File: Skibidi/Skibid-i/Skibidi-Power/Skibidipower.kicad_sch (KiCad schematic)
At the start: 19 parts, among them J1 SparkOut, J2 Bat2, J3 Bat1, J5 Sparkout 48V, J6 Sparkin, Q1 SQM40P10-40L_GE3, Q2 SQ2318AES-T1_BE3

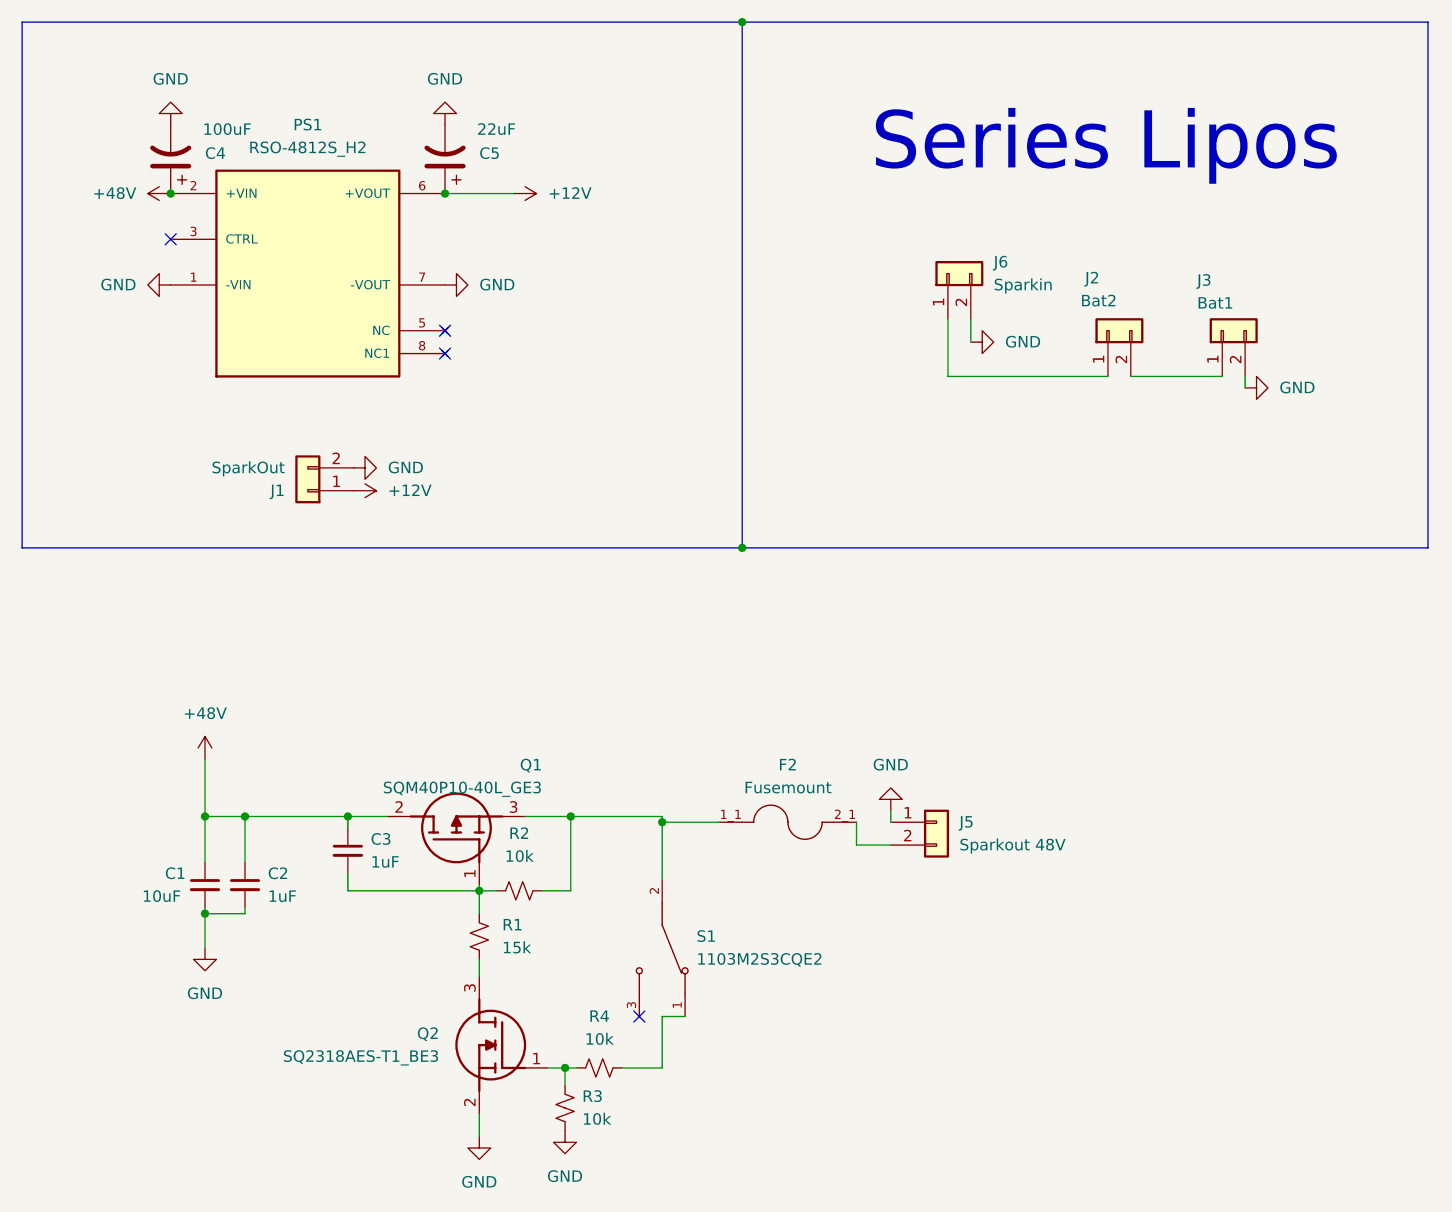
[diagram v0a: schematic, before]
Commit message: pushsuskibnbiid
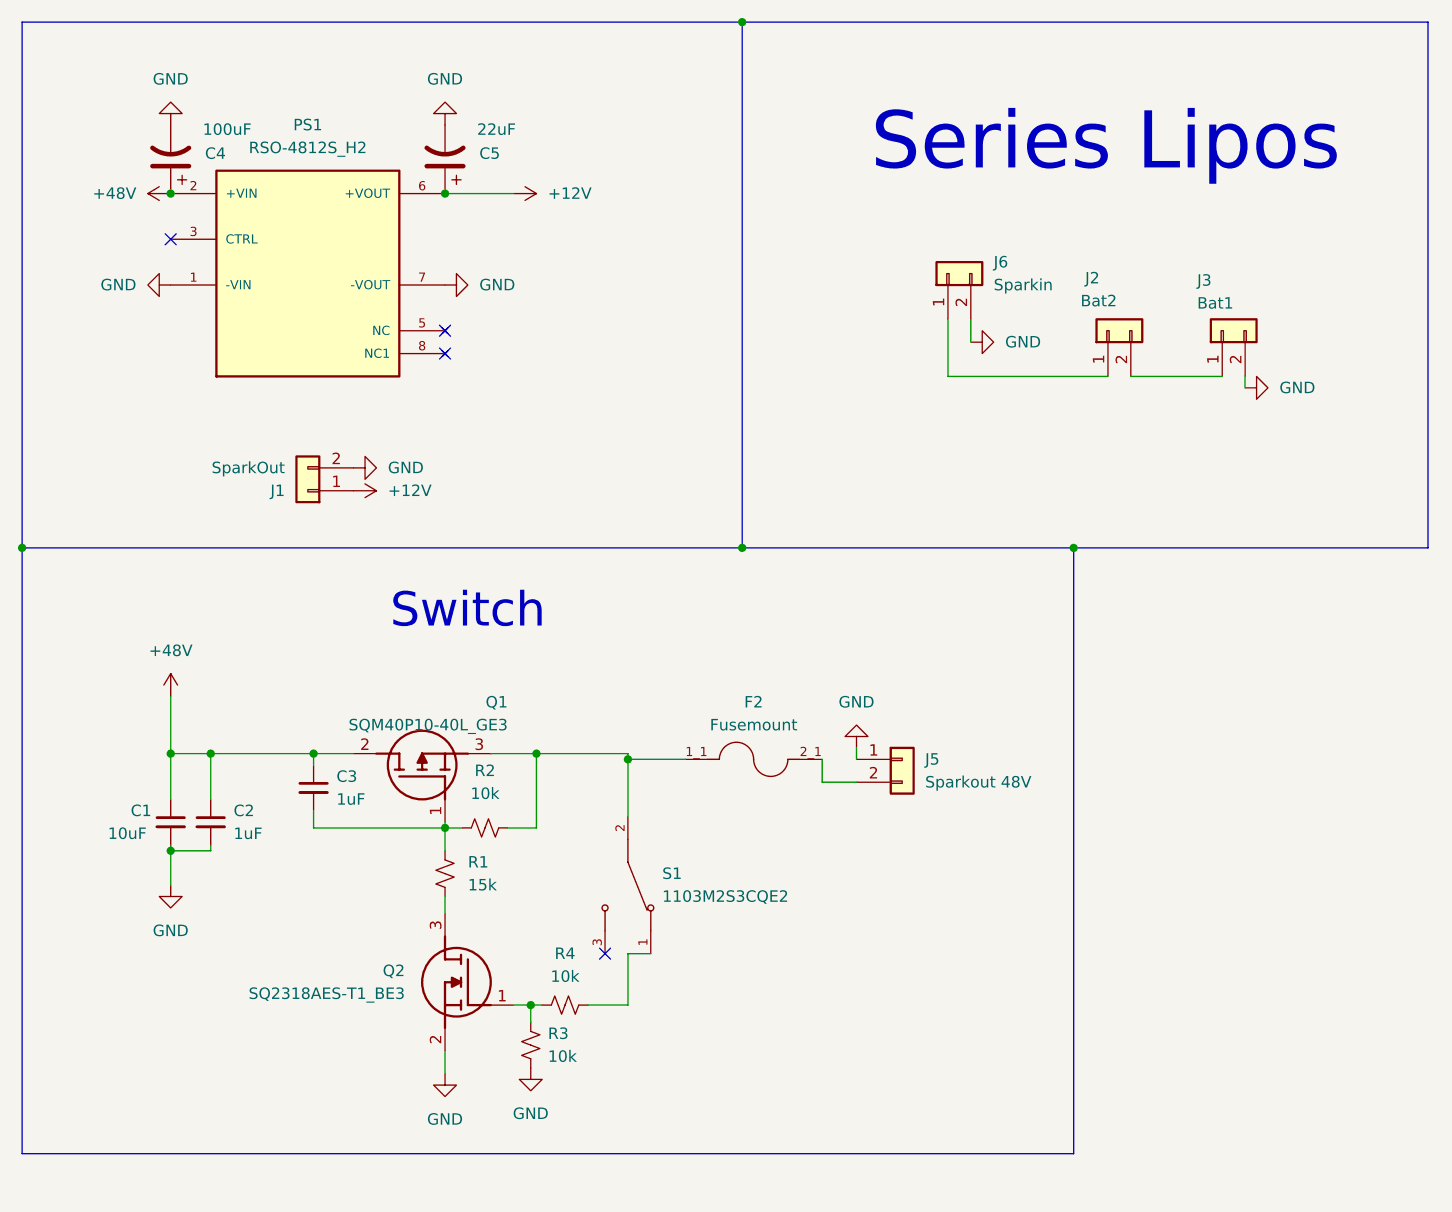
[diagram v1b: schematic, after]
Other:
- note added: "Switch"
- moved on the sheet: C1, C2, C3, F2, J5, Q1, Q2, R1, R2, R3, R4, S1
